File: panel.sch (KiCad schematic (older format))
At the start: 1 part, among them U1 led-panel-16x16

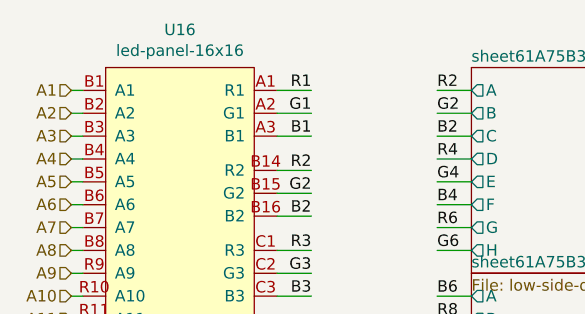
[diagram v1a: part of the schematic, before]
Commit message: Add 16MHz crystal
Turns out the STM32F7 DFU bootloader uses the HSE for USB clocking and
thus requires a crystal. No fallback to HSI is implemented. *sigh*
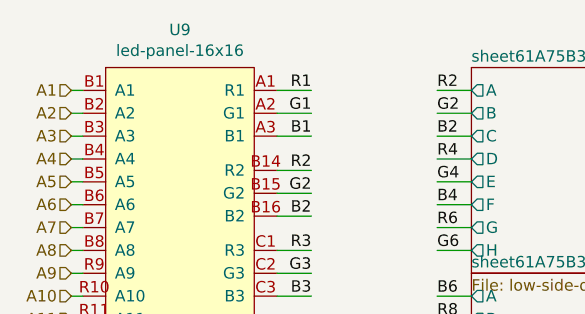
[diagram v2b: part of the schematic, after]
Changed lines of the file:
@@
 $Descr A4 11693 8268
 encoding utf-8
-Sheet 2 25
+Sheet 10 25
 Title ""
 Date ""
@@
 AR Path="/61C4C20D/61A429F9" Ref="U9"  Part="1"
 AR Path="/61C4C905/61A429F9" Ref="U16"  Part="1"
-F 0 "U16" H 3625 6915 50  0000 C CNN
+F 0 "U9" H 3625 6915 50  0000 C CNN
 F 1 "led-panel-16x16" H 3625 6824 50  0000 C CNN
 F 2 "led-panel:bga-led-panel-16x16" H 3400 6800 50  0001 C CNN

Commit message: Make space for STM32
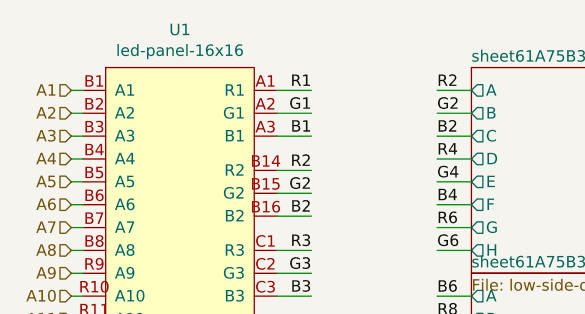
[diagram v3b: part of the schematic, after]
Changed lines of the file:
@@
 $Descr A4 11693 8268
 encoding utf-8
-Sheet 10 25
+Sheet 2 25
 Title ""
 Date ""
@@
 AR Path="/61C4C20D/61A429F9" Ref="U9"  Part="1"
 AR Path="/61C4C905/61A429F9" Ref="U16"  Part="1"
-F 0 "U9" H 3625 6915 50  0000 C CNN
+F 0 "U1" H 3625 6915 50  0000 C CNN
 F 1 "led-panel-16x16" H 3625 6824 50  0000 C CNN
 F 2 "led-panel:bga-led-panel-16x16" H 3400 6800 50  0001 C CNN

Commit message: Add tag connect programming/debug interface
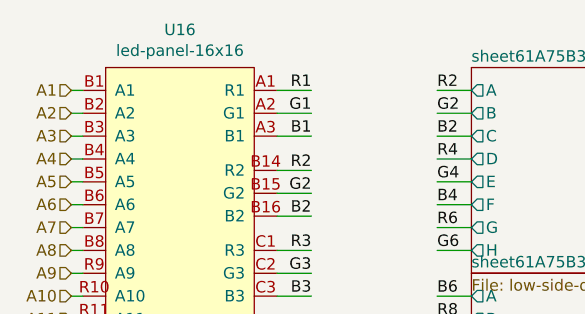
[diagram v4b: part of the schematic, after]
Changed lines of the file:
@@
 $Descr A4 11693 8268
 encoding utf-8
-Sheet 2 25
+Sheet 17 25
 Title ""
 Date ""
@@
 AR Path="/61C4C20D/61A429F9" Ref="U9"  Part="1"
 AR Path="/61C4C905/61A429F9" Ref="U16"  Part="1"
-F 0 "U1" H 3625 6915 50  0000 C CNN
+F 0 "U16" H 3625 6915 50  0000 C CNN
 F 1 "led-panel-16x16" H 3625 6824 50  0000 C CNN
 F 2 "led-panel:bga-led-panel-16x16" H 3400 6800 50  0001 C CNN
